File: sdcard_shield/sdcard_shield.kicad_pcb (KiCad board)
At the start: 2 copper layers, 25.5 x 25.4 mm, 5 parts, among them J1 esp_23-5, J2 sd_reader, J3 PWR

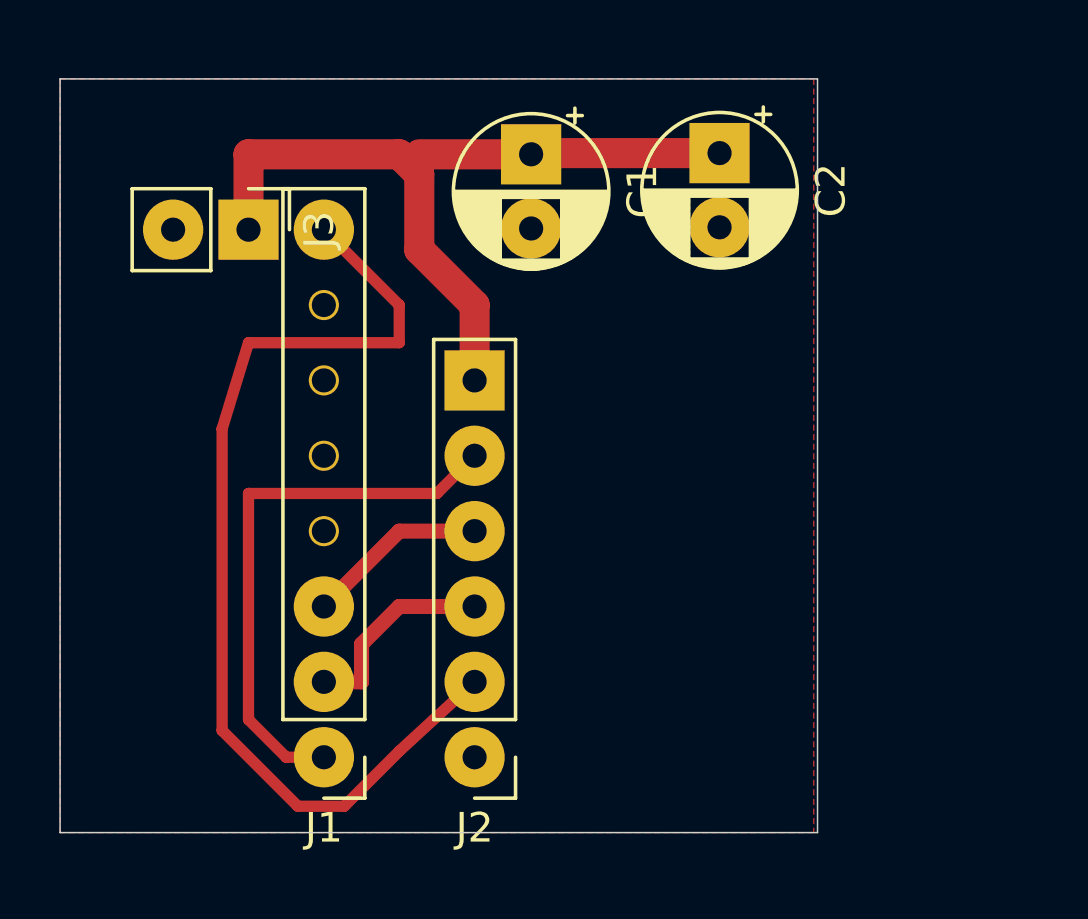
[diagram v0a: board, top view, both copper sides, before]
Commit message: fixed it
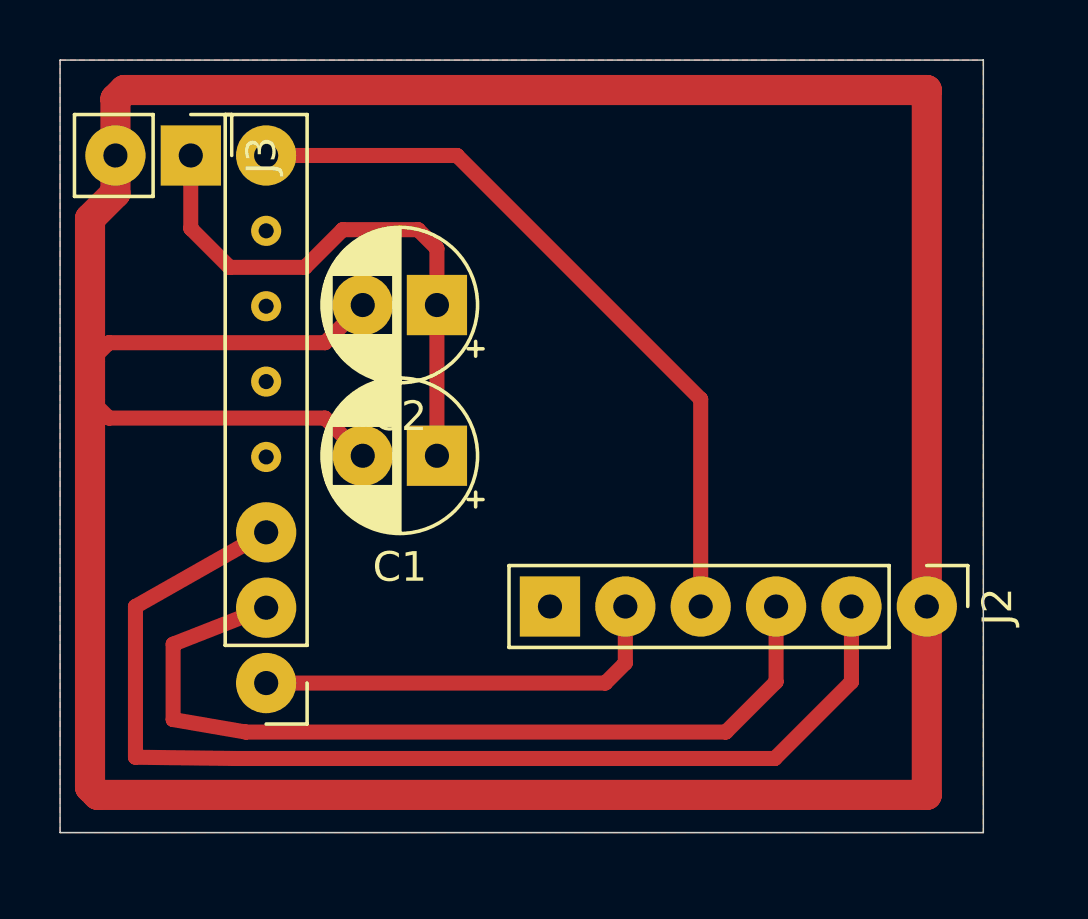
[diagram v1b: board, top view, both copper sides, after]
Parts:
- moved J2 16.1 mm to (29.2, 17.8), turned to -90 degrees
- moved C2 10.8 mm to (12.7, 7.62), turned to 180 degrees
- moved C1 10.6 mm to (12.7, 12.7), turned to 180 degrees
- moved J1 3.17 mm to (6.95, 20.4)
- moved J3 3.17 mm to (4.41, 2.58)
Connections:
- J1 pad 3: MOSI -> MISO
- J1 pad 8: MISO -> MOSI
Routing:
- net G: track 0.00 -> 123.0 mm
- net CLK: track 6.88 -> 29.5 mm
- net MOSI: track 6.13 -> 25.0 mm
- net 3V3: track 26.4 -> 20.0 mm
- net CS: track 18.8 -> 14.3 mm
- net MISO: track 34.4 -> 37.9 mm
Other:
- board size 25.5 x 25.4 mm -> 31.1 x 26 mm

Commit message: dammit. fixed
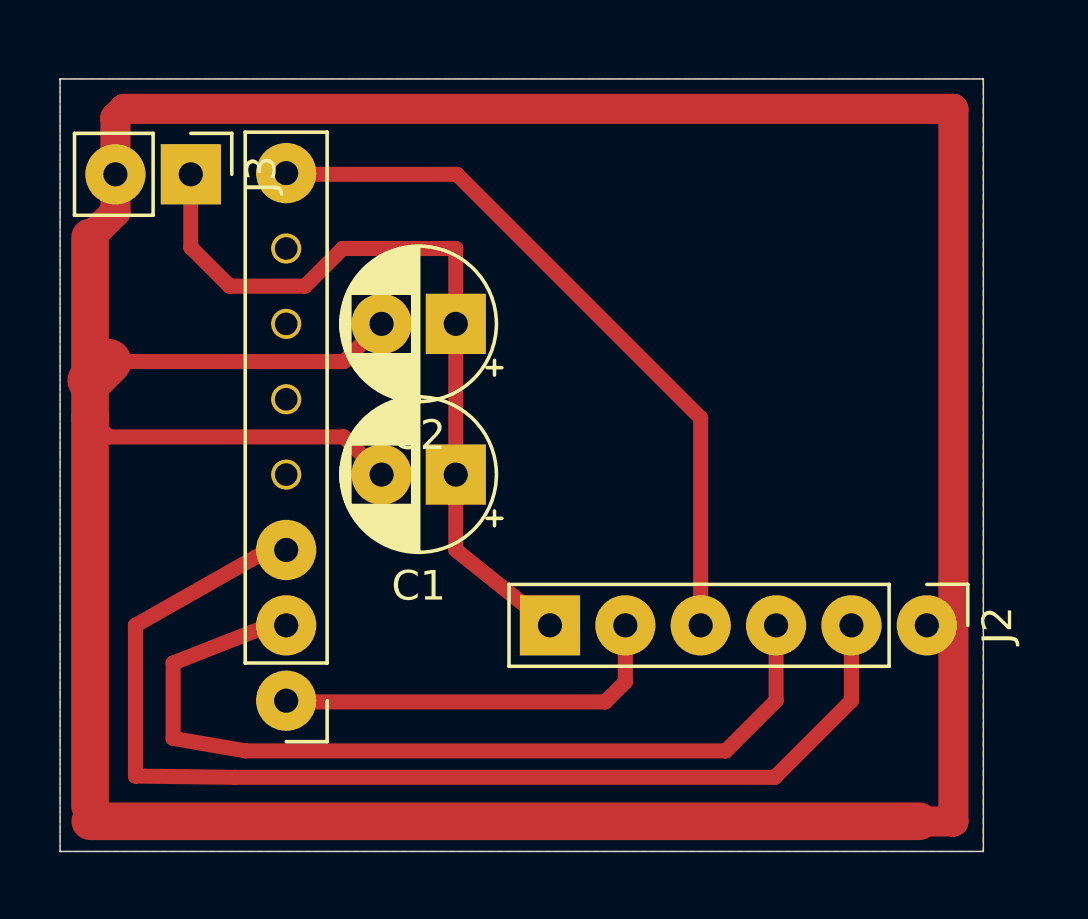
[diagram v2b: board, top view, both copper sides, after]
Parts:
- moved J1 0.90 mm to (7.62, 21.0)
- moved C1 0.90 mm to (13.3, 13.3)
- moved C2 0.90 mm to (13.3, 8.26)
- moved J3 0.63 mm to (4.41, 3.21)
- moved J2 0.63 mm to (29.2, 18.4)
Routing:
- net 3V3: track 20.0 -> 26.7 mm
- net G: track 123.0 -> 127.4 mm
